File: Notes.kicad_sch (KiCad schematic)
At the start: 0 parts

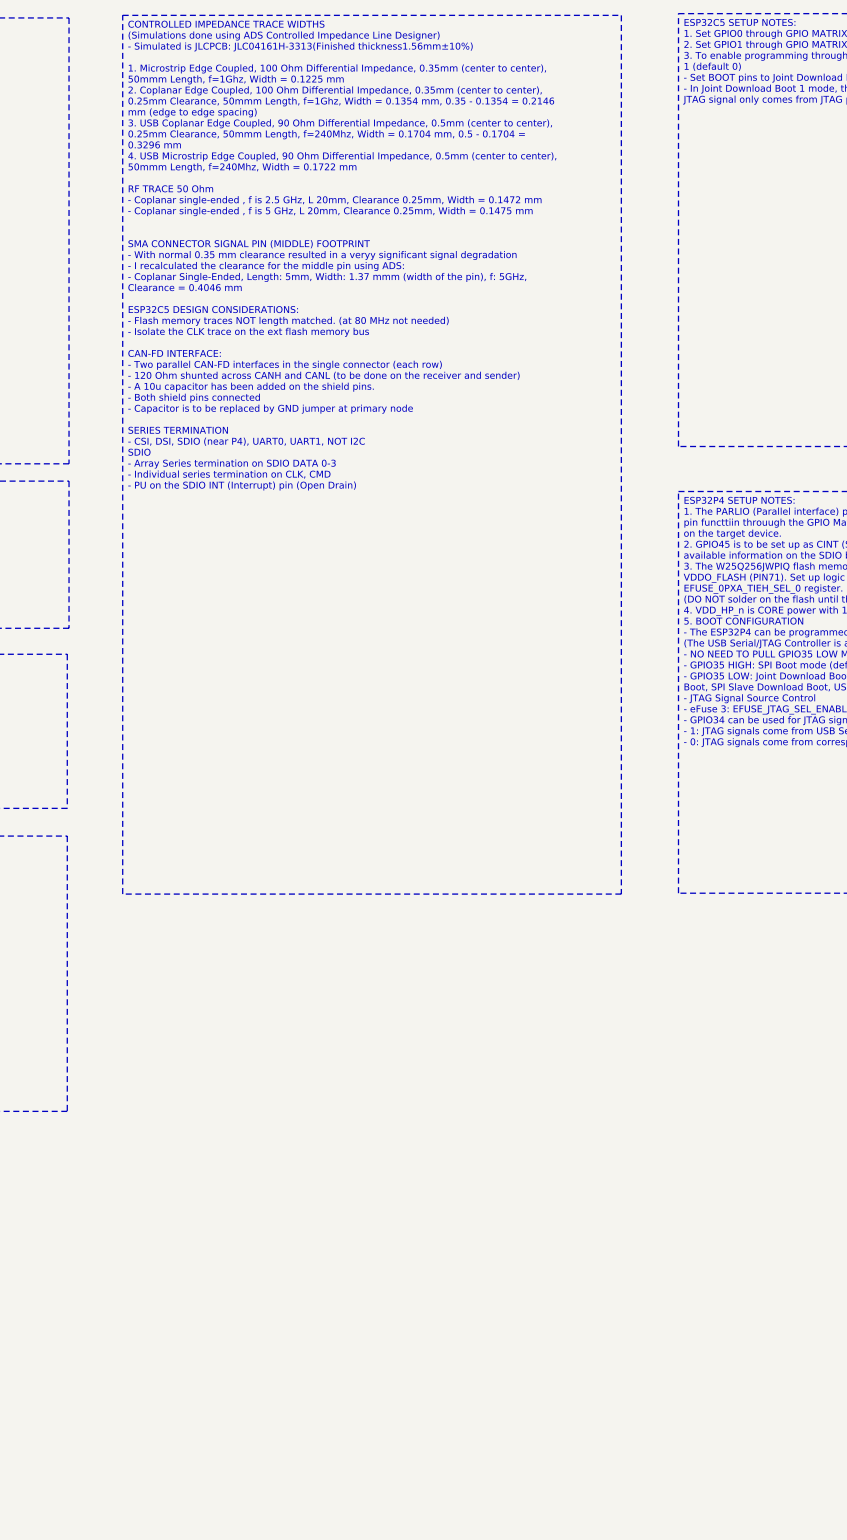
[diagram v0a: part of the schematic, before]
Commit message: C5 RF Update
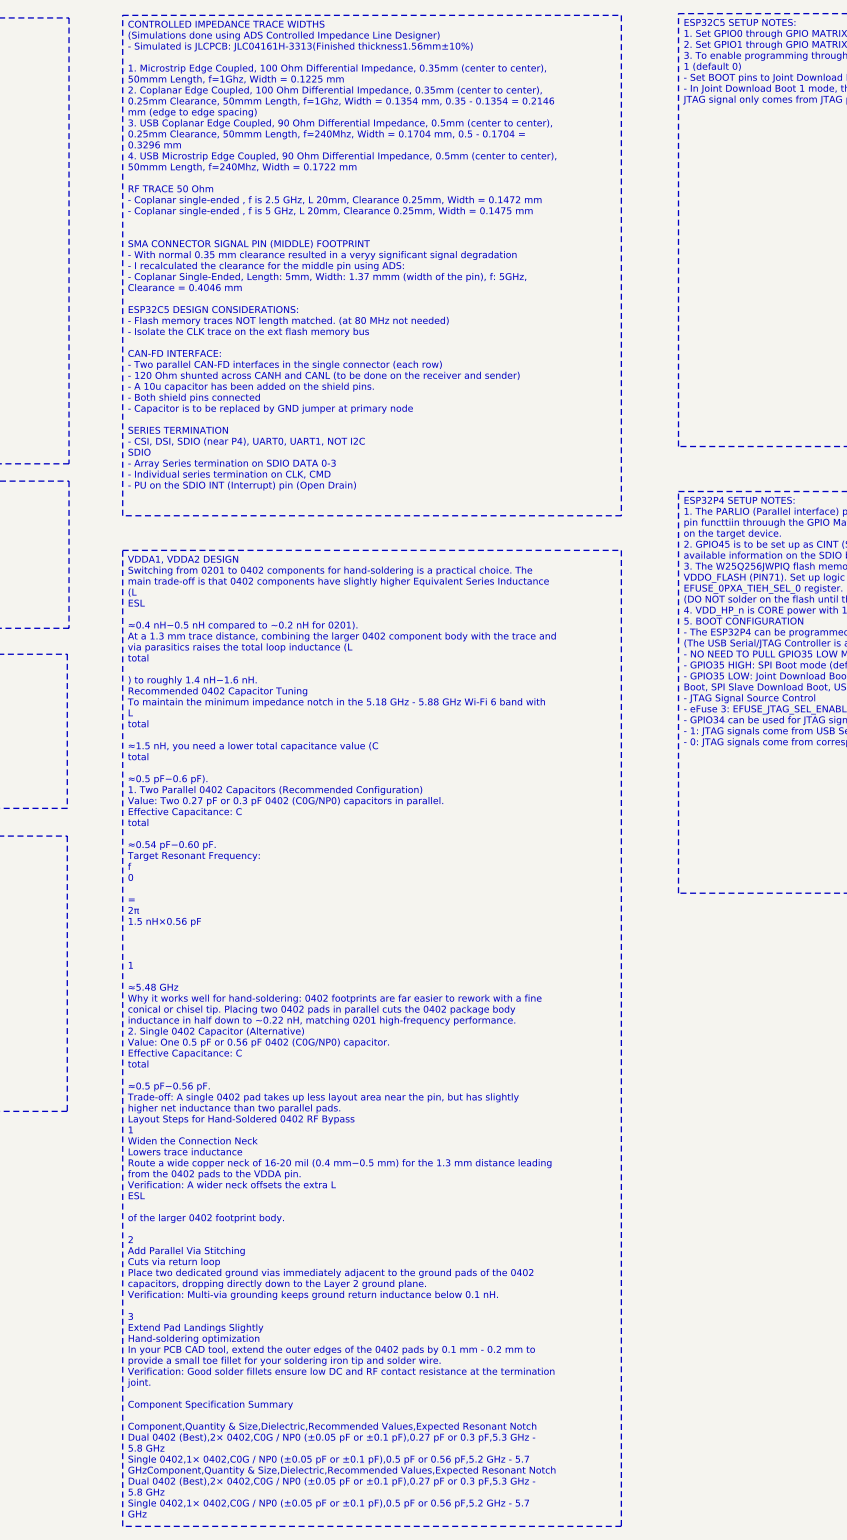
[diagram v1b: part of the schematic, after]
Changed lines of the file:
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@@
 		(exclude_from_sim no)
 		(at 113.03 29.464 0)
-		(size 73.152 128.905)
+		(size 73.152 73.406)
 		(margins 0.75 0.75 0.75 0.75)
 		(stroke
+			(width 0)
+			(type dash)
+		)
+		(fill
+			(type none)
+		)
+		(effects
+			(font
+				(size 1 1)
+			)
+			(justify left top)
+		)
+	)
+	(text_box "VDDA1, VDDA2 DESIGN\nSwitching from 0201 to 0402 components for hand-soldering is a practical choice. The main trade-off is that 0402 components have slightly higher Equivalent Series Inductance (L \nESL\n​	\n ≈0.4 nH−0.5 nH compared to ∼0.2 nH for 0201).\nAt a 1.3 mm trace distance, combining the larger 0402 component body with the trace and via parasitics raises the total loop inductance (L \ntotal\n​	\n ) to roughly 1.4 nH−1.6 nH.\nRecommended 0402 Capacitor Tuning\nTo maintain the minimum impedance notch in the 5.18 GHz - 5.88 GHz Wi-Fi 6 band with L \ntotal\n​	\n ≈1.5 nH, you need a lower total capacitance value (C \ntotal\n​	\n ≈0.5 pF−0.6 pF).\n1. Two Parallel 0402 Capacitors (Recommended Configuration)\nValue: Two 0.27 pF or 0.3 pF 0402 (C0G/NP0) capacitors in parallel.\nEffective Capacitance: C \ntotal\n​	\n ≈0.54 pF−0.60 pF.\nTarget Resonant Frequency:\nf \n0\n​	\n = \n2π \n1.5 nH×0.56 pF\n\n​	\n \n1\n​	\n ≈5.48 GHz\nWhy it works well for hand-soldering: 0402 footprints are far easier to rework with a fine conical or chisel tip. Placing two 0402 pads in parallel cuts the 0402 package body inductance in half down to ∼0.22 nH, matching 0201 high-frequency performance.\n2. Single 0402 Capacitor (Alternative)\nValue: One 0.5 pF or 0.56 pF 0402 (C0G/NP0) capacitor.\nEffective Capacitance: C \ntotal\n​	\n ≈0.5 pF−0.56 pF.\nTrade-off: A single 0402 pad takes up less layout area near the pin, but has slightly higher net inductance than two parallel pads.\nLayout Steps for Hand-Soldered 0402 RF Bypass\n1\nWiden the Connection Neck\nLowers trace inductance\nRoute a wide copper neck of 16-20 mil (0.4 mm−0.5 mm) for the 1.3 mm distance leading from the 0402 pads to the VDDA pin.\nVerification: A wider neck offsets the extra L \nESL\n​	\n  of the larger 0402 footprint body.\n\n2\nAdd Parallel Via Stitching\nCuts via return loop\nPlace two dedicated ground vias immediately adjacent to the ground pads of the 0402 capacitors, dropping directly down to the Layer 2 ground plane.\nVerification: Multi-via grounding keeps ground return inductance below 0.1 nH.\n\n3\nExtend Pad Landings Slightly\nHand-soldering optimization\nIn your PCB CAD tool, extend the outer edges of the 0402 pads by 0.1 mm - 0.2 mm to provide a small toe fillet for your soldering iron tip and solder wire.\nVerification: Good solder fillets ensure low DC and RF contact resistance at the termination joint.\n\nComponent Specification Summary\n\nComponent,Quantity & Size,Dielectric,Recommended Values,Expected Resonant Notch\nDual 0402 (Best),2× 0402,C0G / NP0 (±0.05 pF or ±0.1 pF),0.27 pF or 0.3 pF,5.3 GHz - 5.8 GHz\nSingle 0402,1× 0402,C0G / NP0 (±0.05 pF or ±0.1 pF),0.5 pF or 0.56 pF,5.2 GHz - 5.7 GHzComponent,Quantity & Size,Dielectric,Recommended Values,Expected Resonant Notch\nDual 0402 (Best),2× 0402,C0G / NP0 (±0.05 pF or ±0.1 pF),0.27 pF or 0.3 pF,5.3 GHz - 5.8 GHz\nSingle 0402,1× 0402,C0G / NP0 (±0.05 pF or ±0.1 pF),0.5 pF or 0.56 pF,5.2 GHz - 5.7 GHz"
+		(exclude_from_sim no)
+		(at 113.03 107.95 0)
+		(size 73.152 143.1739)
+		(margins 0.75 0.75 0.75 0.75)
+		(stroke

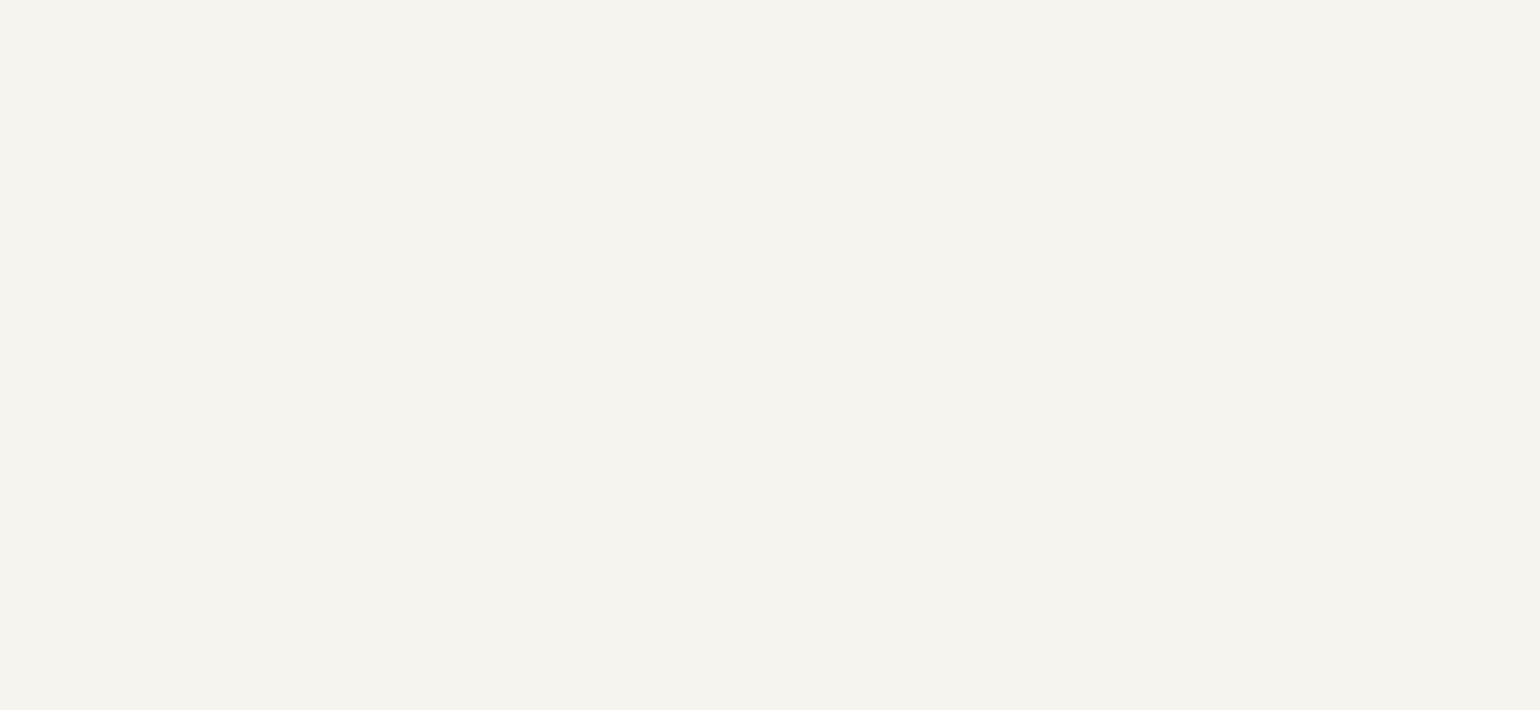
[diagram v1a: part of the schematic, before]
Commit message: RF Update
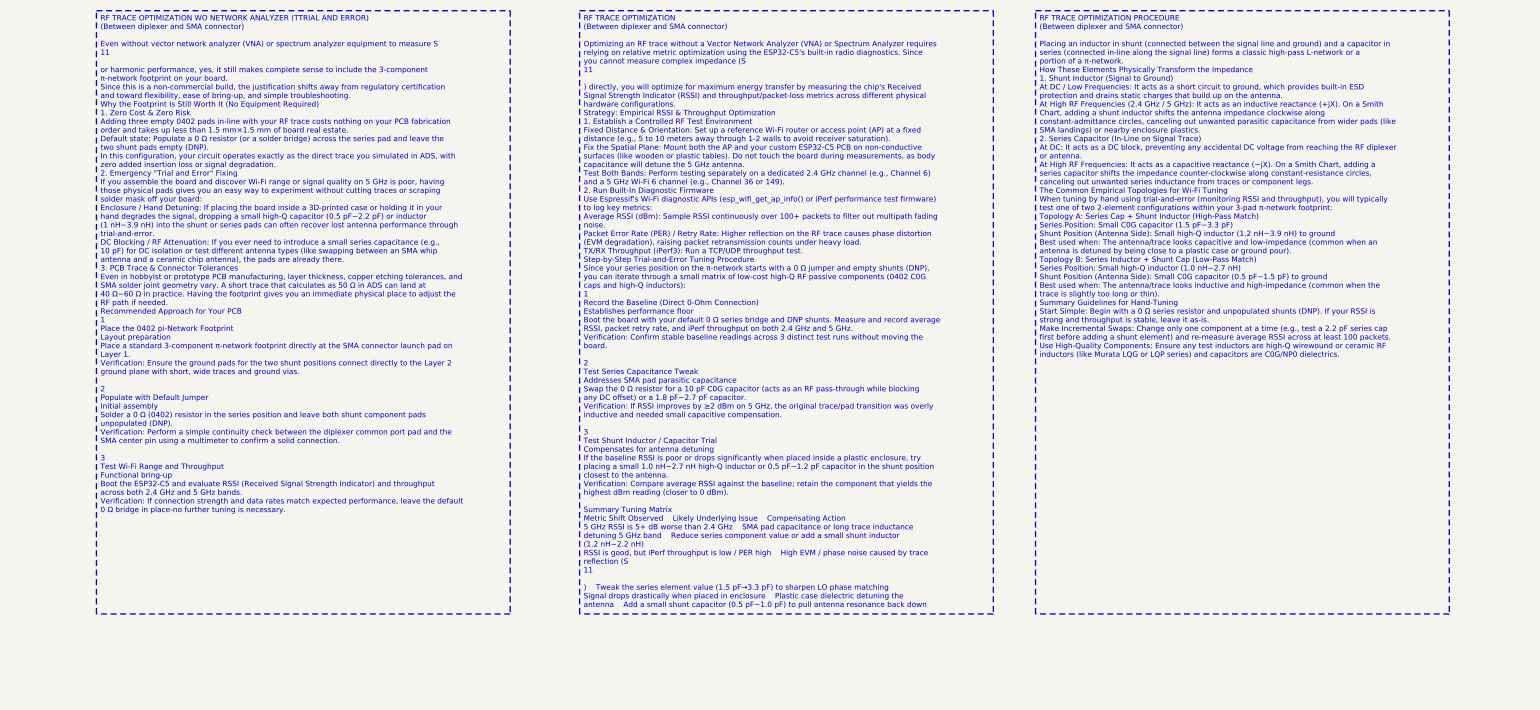
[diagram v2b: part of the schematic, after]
